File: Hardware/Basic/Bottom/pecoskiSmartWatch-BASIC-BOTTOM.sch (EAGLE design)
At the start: 32 parts

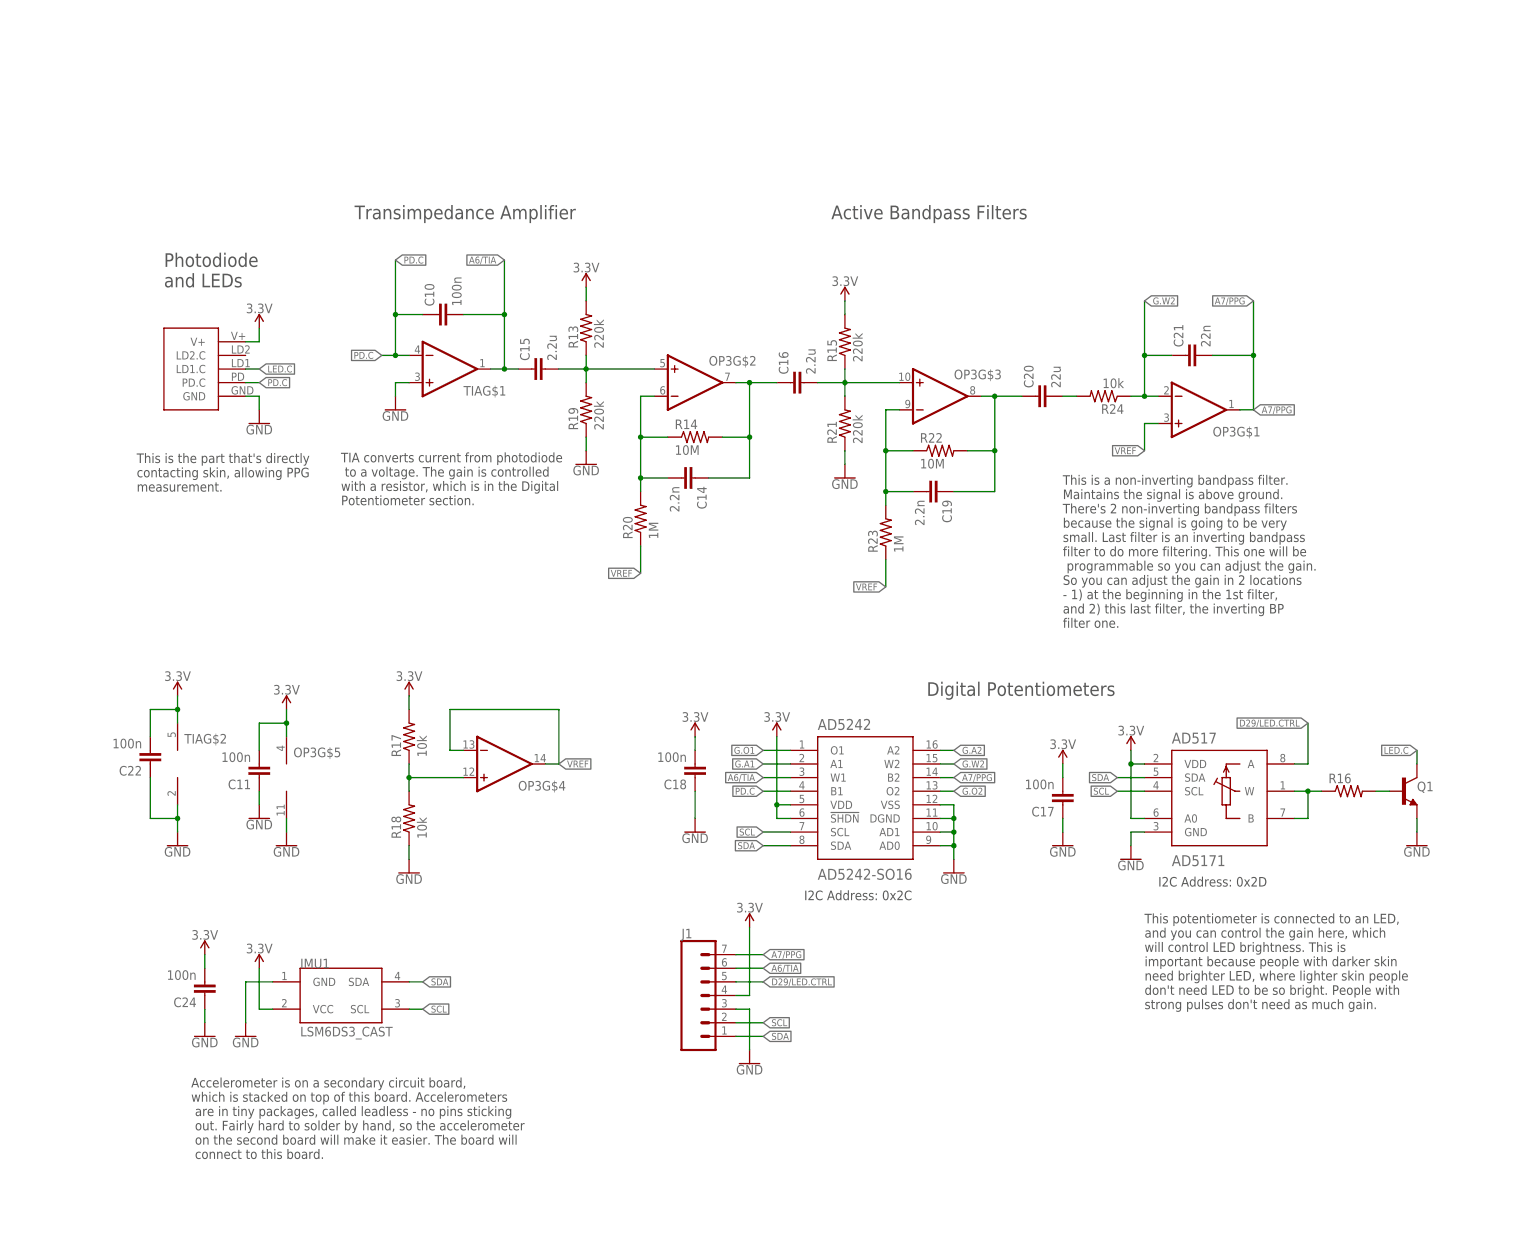
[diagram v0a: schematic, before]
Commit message: HW Updates 2021/03/06
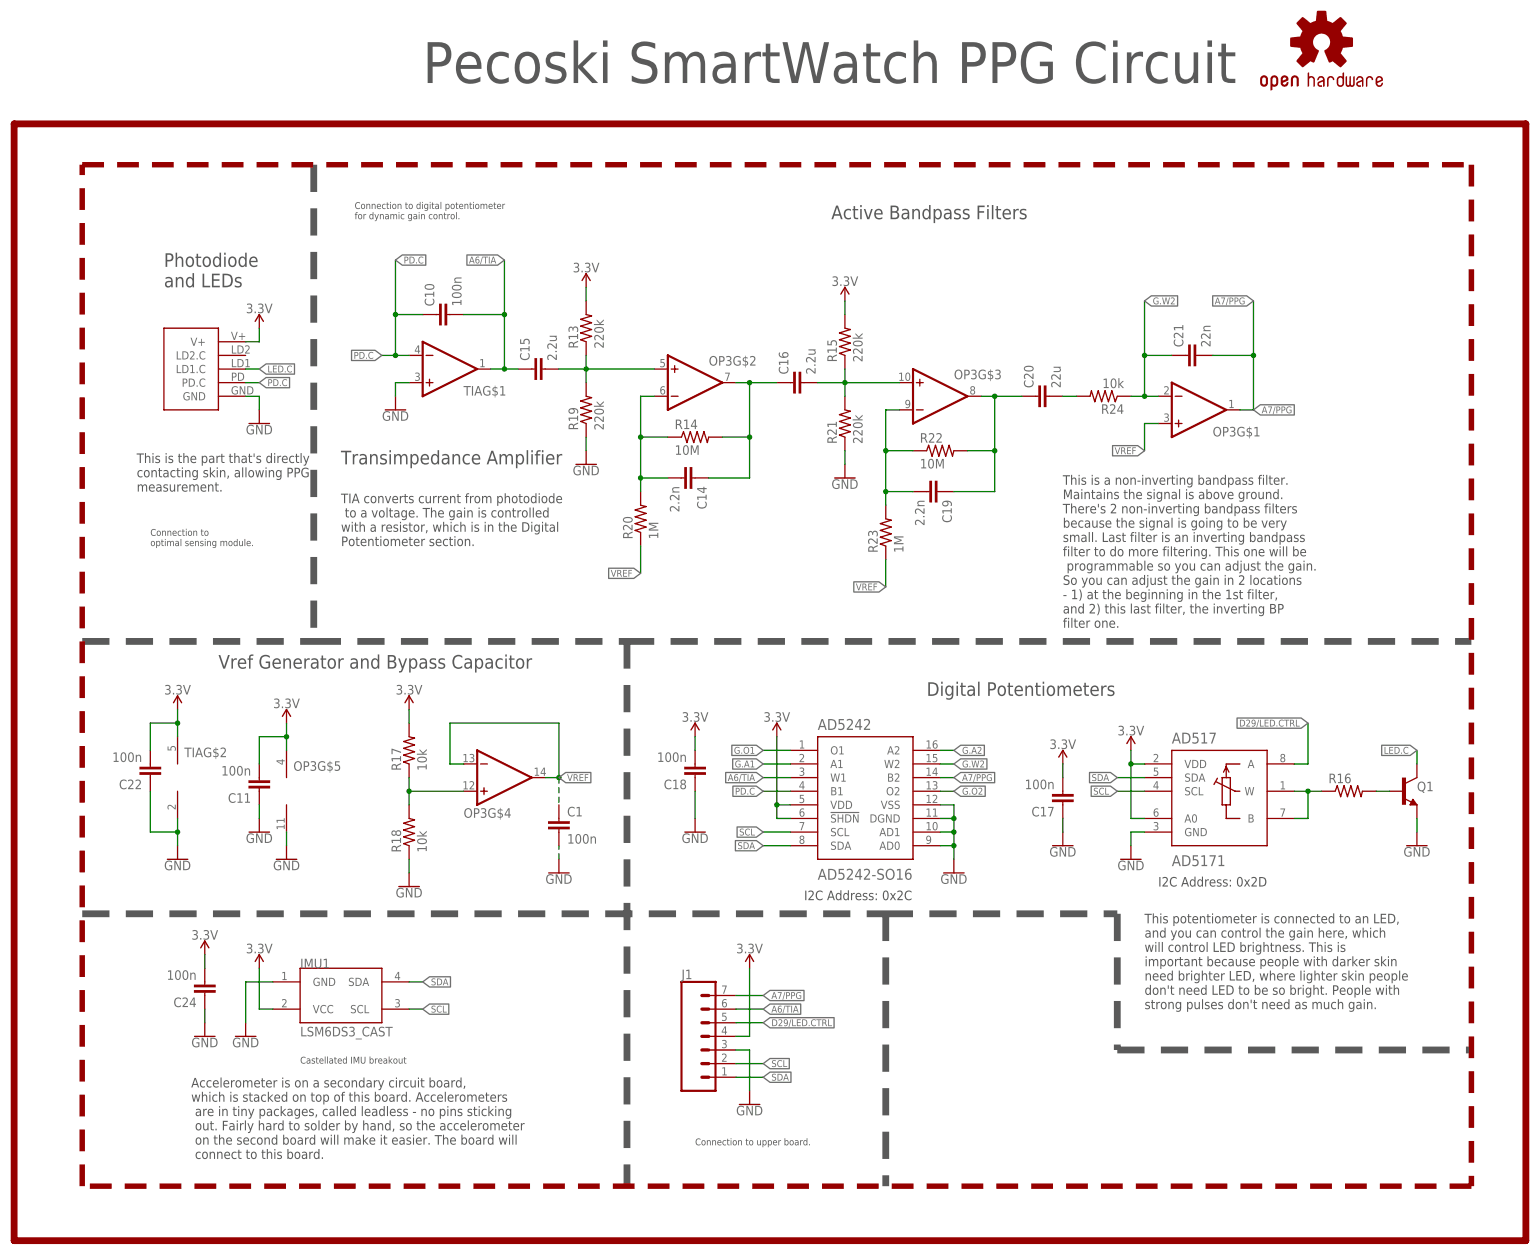
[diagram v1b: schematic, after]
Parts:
- added C1: 100n, LinnesLab-Passives:CAPACITOR0603
- added LOGO1: REVISION.A, LinnesLab-Logos:REVISION.A
- added LOGO2: OSHW-LOGOS, LinnesLab-Logos:OSHW-LOGOS
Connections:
- net GND: now also C1.2
- net VREF: now also C1.1
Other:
- note added: "Castellated IMU breakout"
- note added: "Connection to digital potentiometer for dynamic gain control."
- note added: "Connection to optimal sensing module."
- note added: "Connection to upper board."
- note added: "Pecoski SmartWatch PPG Circuit"
- note added: "Vref Generator and Bypass Capacitor"
- moved on the sheet: C11, C22, J1, OP3G$4, OP3G$5, R17, R18, TIAG$2
